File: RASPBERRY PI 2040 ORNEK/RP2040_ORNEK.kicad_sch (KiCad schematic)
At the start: 34 parts, among them J1 USB_B_Micro, J2 Conn_01x02, J3 Conn_02x18_Odd_Even, J4 Conn_02x18_Odd_Even, U1 NCP1117-3.3_SOT223, U2 W25Q128JVS, U3 RP2040, Y1 ABLS-12.000MHZ-B4-T

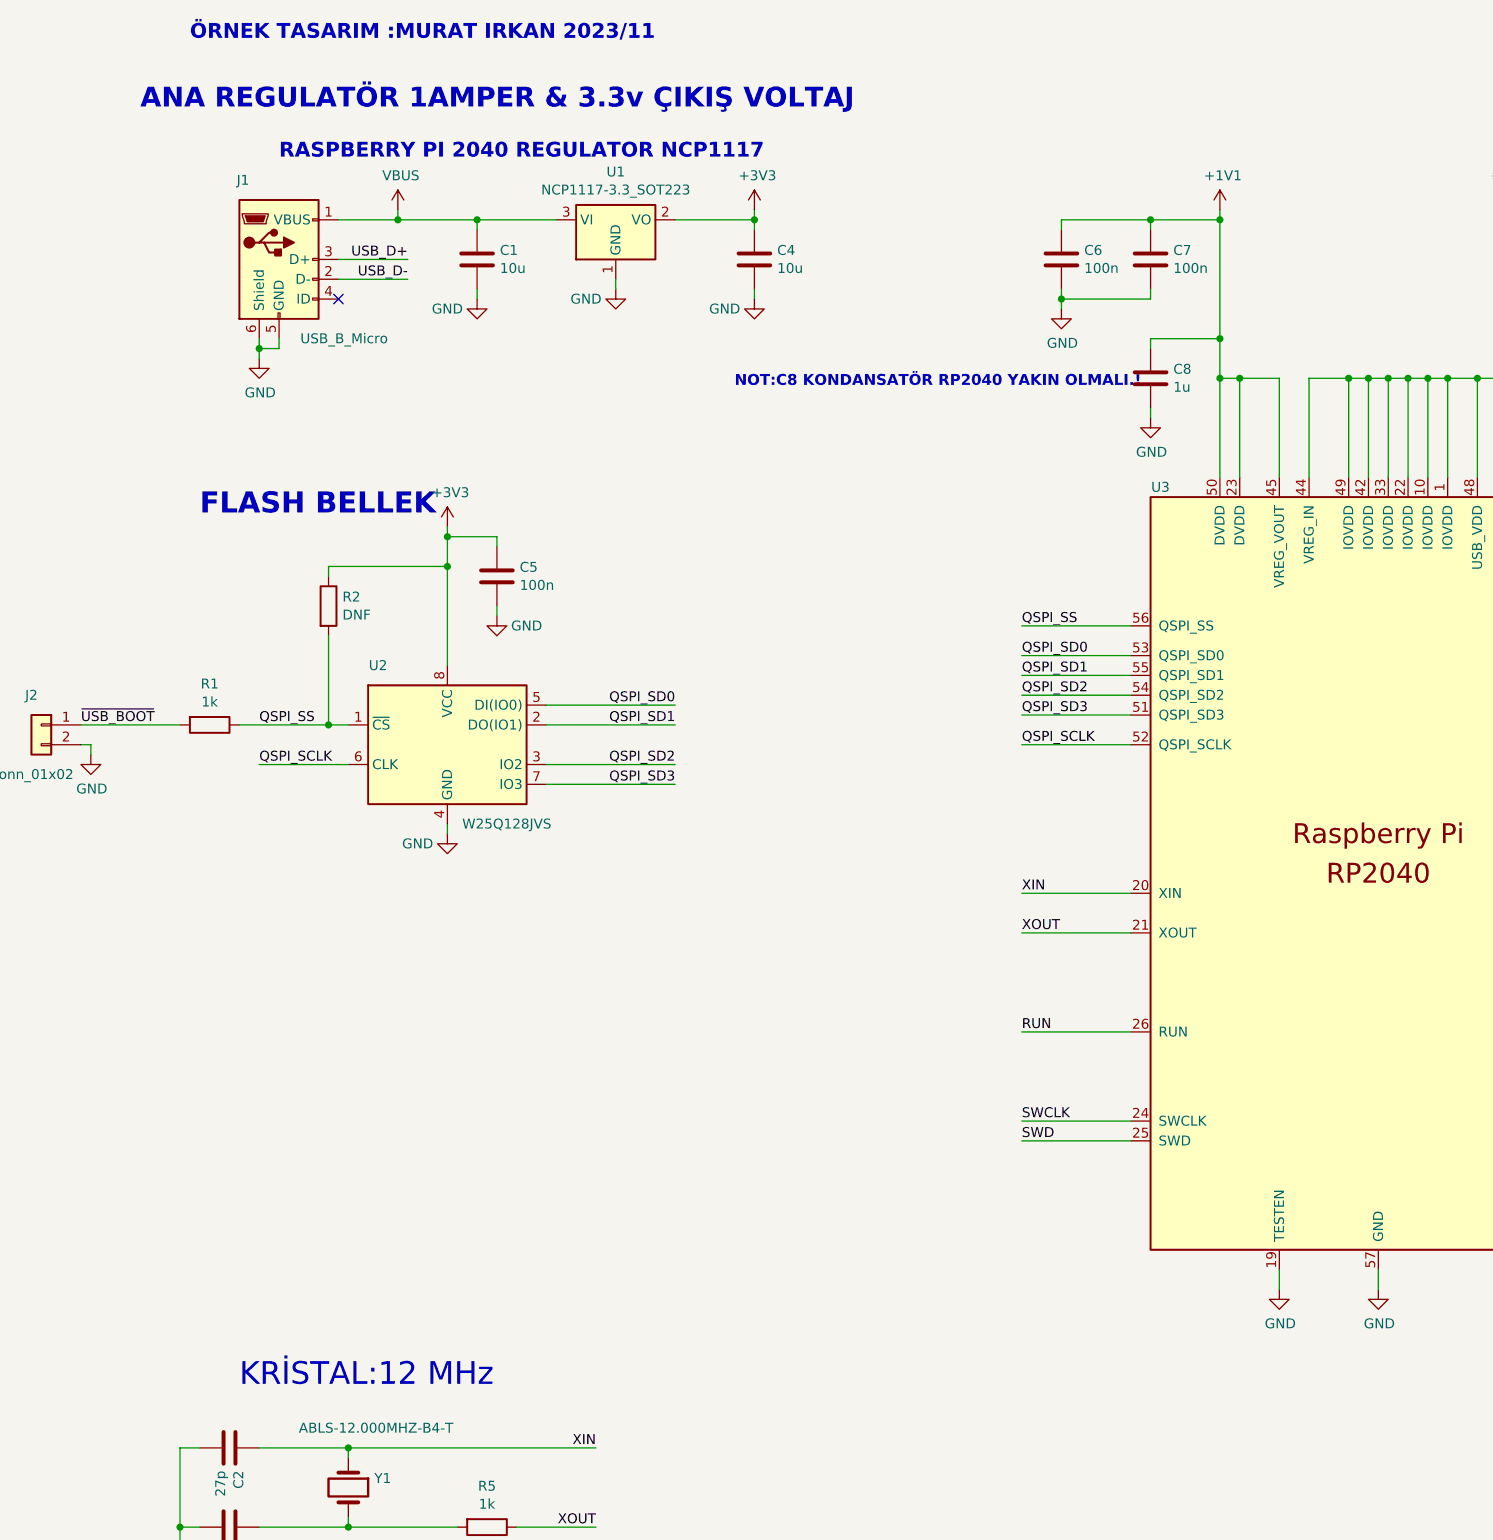
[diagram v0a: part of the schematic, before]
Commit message: RASPBERRY PI 2040 ÖRNEK TASARIM: REV.1.01
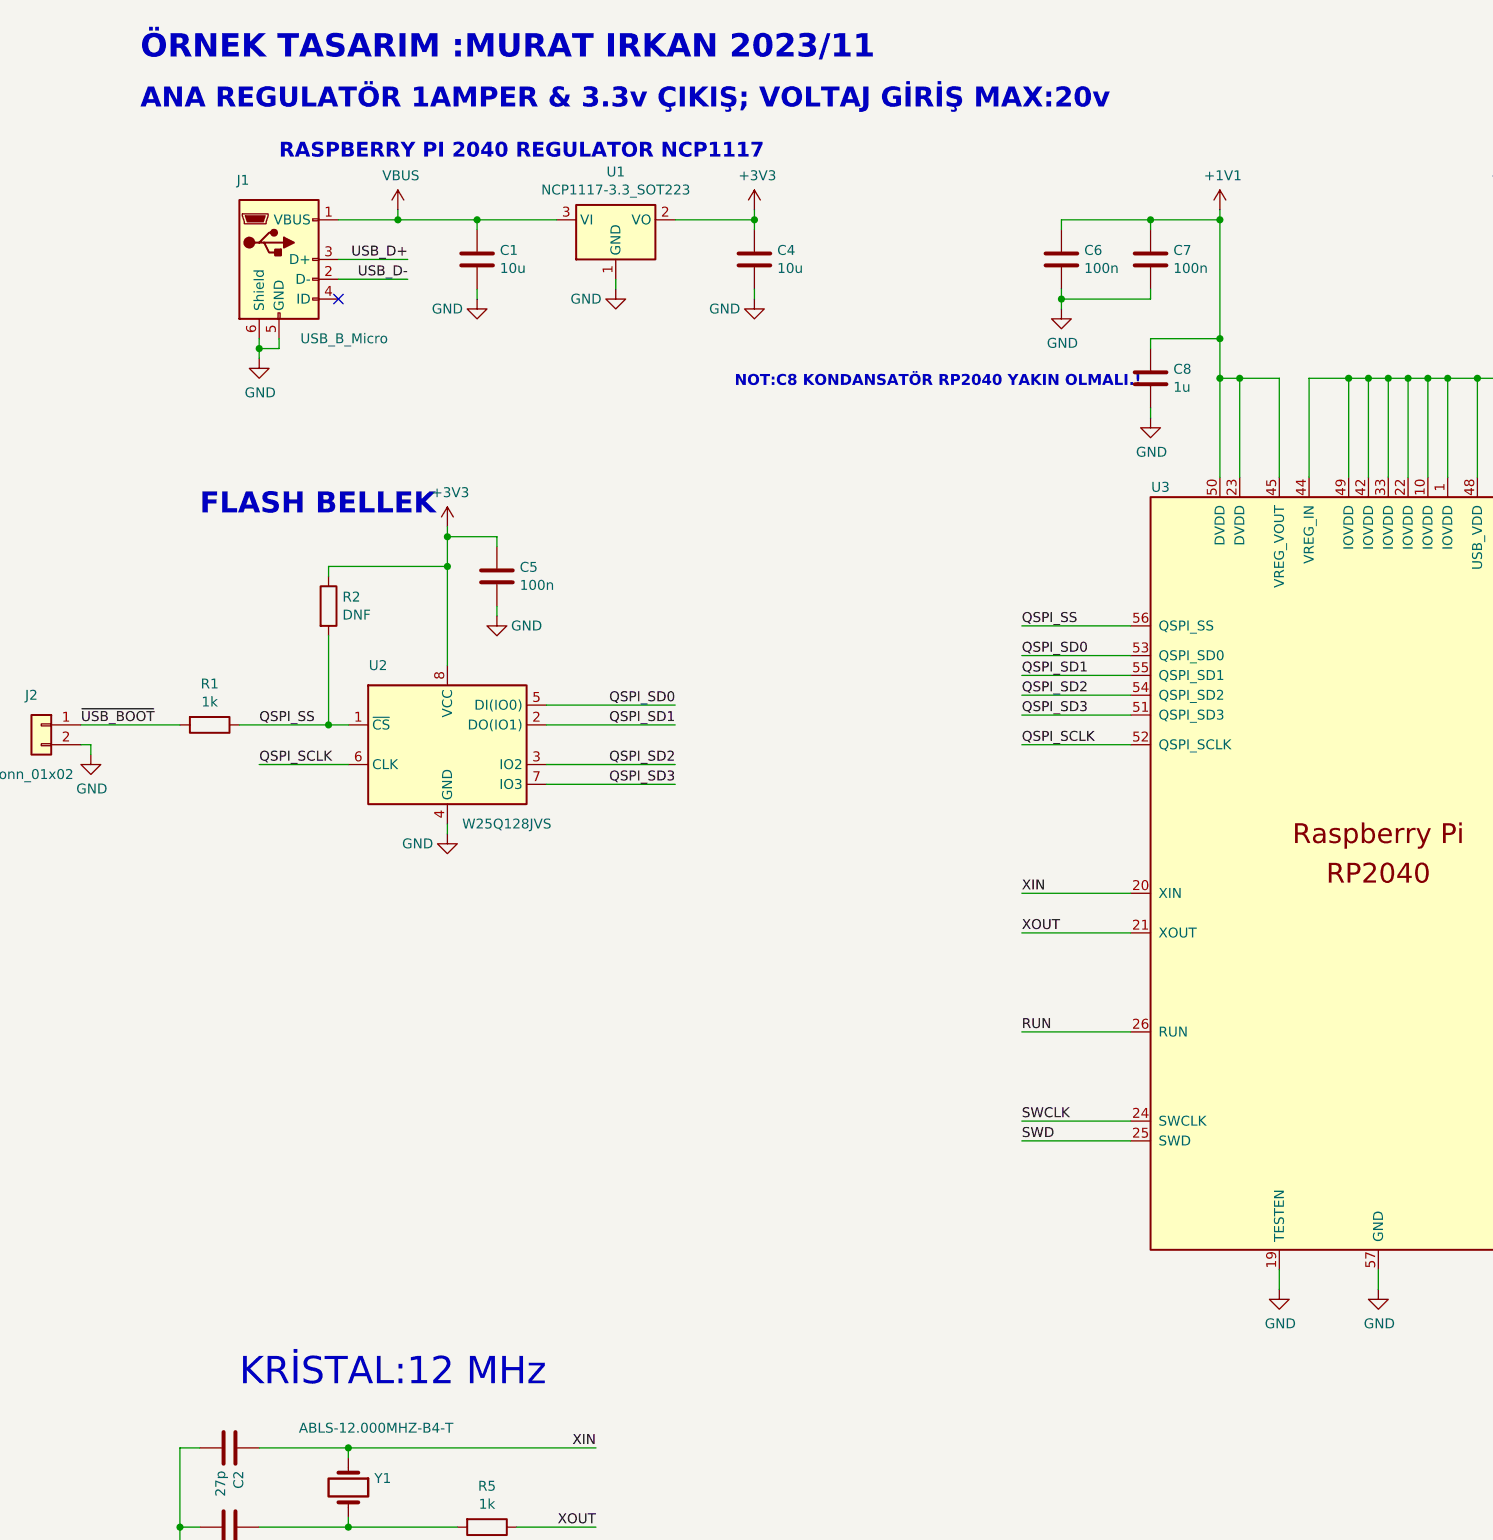
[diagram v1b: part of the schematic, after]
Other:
- note added: "ANA REGULATÖR 1AMPER & 3.3v ÇIKIŞ; VOLTAJ GİRİŞ MAX:20v"
- note removed: "ANA REGULATÖR 1AMPER & 3.3v ÇIKIŞ VOLTAJ"
